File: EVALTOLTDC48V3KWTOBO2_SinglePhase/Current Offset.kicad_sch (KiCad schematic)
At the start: 8 parts

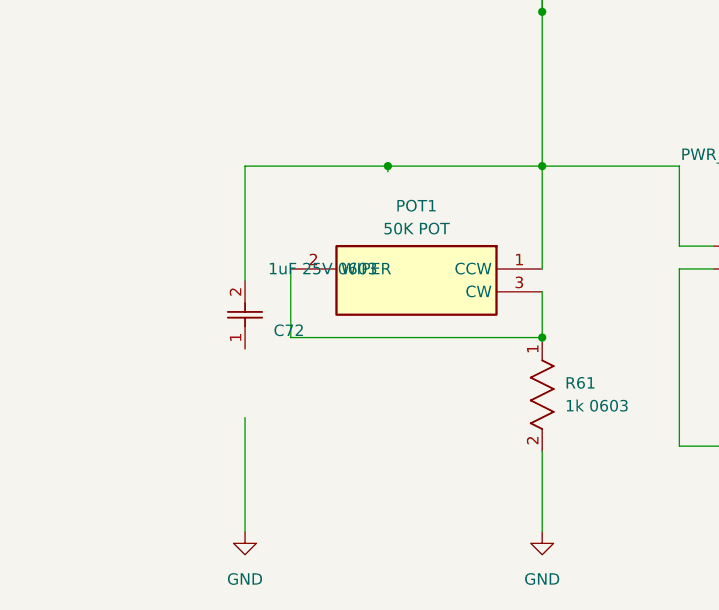
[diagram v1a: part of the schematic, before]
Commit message: Change 4
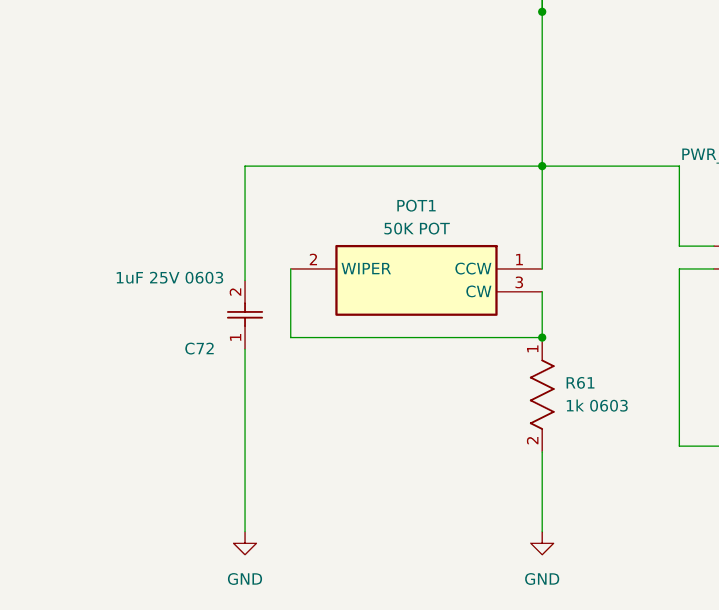
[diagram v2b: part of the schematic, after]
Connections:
- net GND: now also C72.1
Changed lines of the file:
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@@
-	)
-	(junction
-		(at 71.755 63.5)
-		(diameter 0)
-		(color 0 0 0 0)
 	)
 	(junction
@@
 	(wire
 		(pts
-			(xy 88.9 63.5) (xy 71.755 63.5)
+			(xy 55.88 63.5) (xy 88.9 63.5)
 		)
 		(stroke
@@
 	(wire
 		(pts
-			(xy 55.88 91.44) (xy 55.88 104.14)
+			(xy 55.88 83.82) (xy 55.88 104.14)
 		)
 		(stroke
@@
 	(wire
 		(pts
-			(xy 71.755 64.135) (xy 71.755 63.5)
-		)
-		(stroke
-			(width 0)
-			(type default)
-		)
-	)
-	(wire
-		(pts
 			(xy 116.84 50.165) (xy 135.89 50.165)
 		)
@@
 		(pts
 			(xy 135.89 73.66) (xy 135.89 94.615)
-		)
-		(stroke
-			(width 0)
-			(type default)
-		)
-	)
-	(wire
-		(pts
-			(xy 71.755 63.5) (xy 55.88 63.5)
 		)
 		(stroke
@@
 		(dnp no)
 		(property "Reference" "C72"
-			(at 62.484 81.788 90)
+			(at 52.578 83.82 90)
 			(effects
 				(font
@@
 		)
 		(property "Value" "1uF 25V 0603"
-			(at 70.612 74.93 90)
-			(effects
-				(font
+			(at 53.594 75.946 90)
+			(effects
+				(font
